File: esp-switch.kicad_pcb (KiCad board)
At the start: 2 copper layers, 51.4 x 51.4 mm, 28 parts, among them J1 Screw_Terminal_01x03, J2 Conn_01x04, J4 Conn_01x04, J5 Screw_Terminal_01x02, U1 ATTINY441-SSU, U2 ESP-01v090, U3 MOC3041M, U4 MOC3041M, U5 HLK-PM05

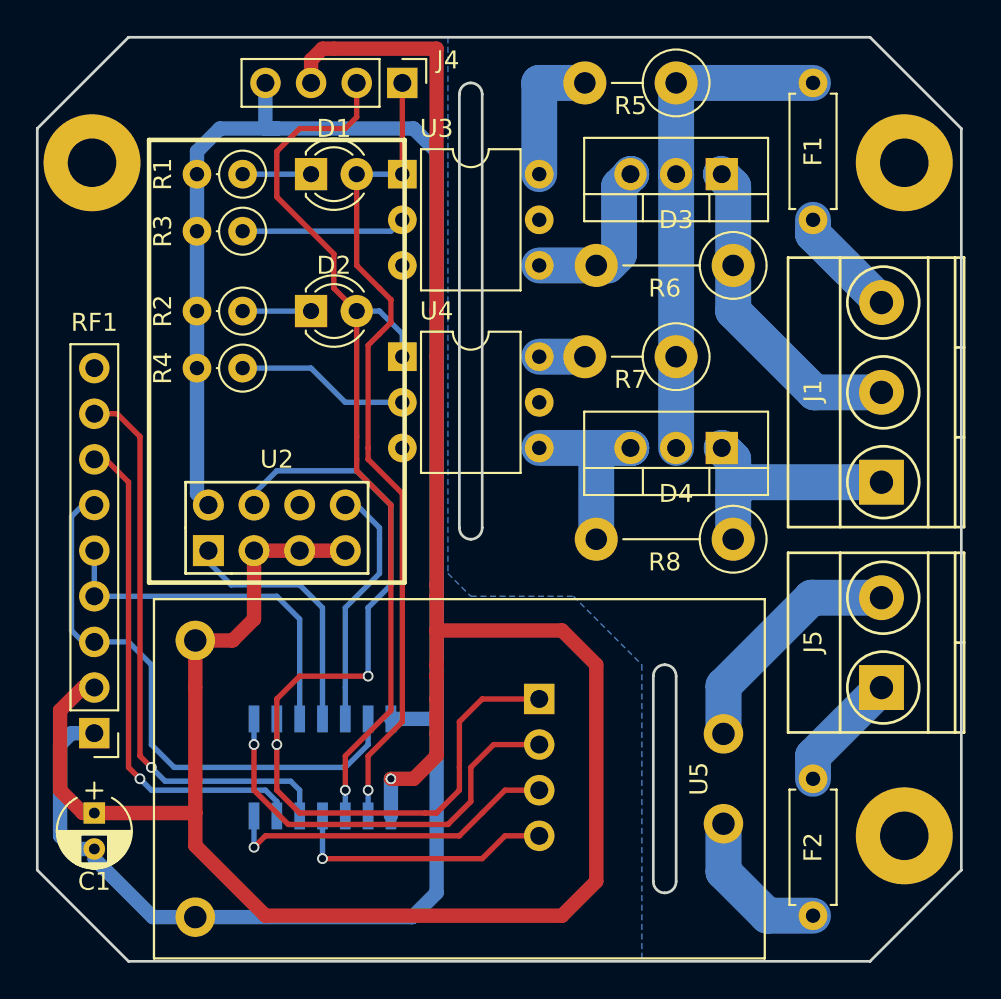
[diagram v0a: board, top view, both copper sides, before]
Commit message: Some changes
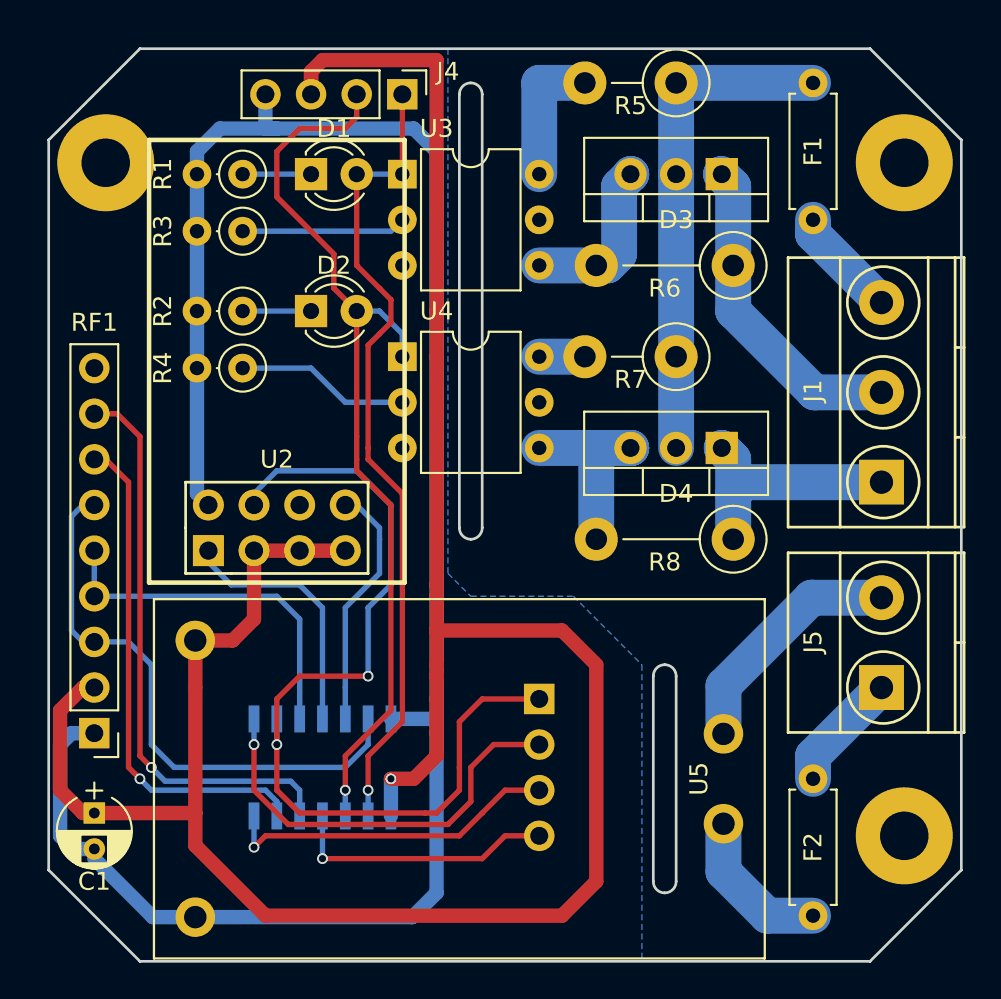
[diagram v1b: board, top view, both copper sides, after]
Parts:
- moved REF** 0.76 mm to (176.5, 99.7)
- moved J4 0.64 mm to (193.0, 95.9)
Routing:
- net Net-(D2-Pad2): track 52.1 -> 51.5 mm
- net Net-(D1-Pad2): track 46.2 -> 45.6 mm
- net GND: track 112.5 -> 111.9 mm
- net +5V: track 139.1 -> 138.5 mm
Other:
- board size 51.4 x 51.4 mm -> 50.8 x 50.8 mm
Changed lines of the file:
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@@
     (area 163.410857 90.20238 240.26 153.195001)
     (thickness 1.6)
-    (drawings 23)
-    (tracks 243)
+    (drawings 21)
+    (tracks 242)
     (zones 0)
     (modules 28)
@@
   )
   (module Mounting_Holes:MountingHole_2.7mm_M2.5_Pad (layer F.Cu)
-    (at 175.768 99.695)
+    (at 176.53 99.695)
     (descr "Mounting Hole 2.7mm, M2.5")
     (tags "mounting hole 2.7mm m2.5")
@@
   )
   (module Pin_Headers:Pin_Header_Straight_1x04_Pitch2.54mm (layer F.Cu)
-    (at 193.04 95.25 270)
+    (at 193.04 95.885 270)
     (descr "Through hole straight pin header, 1x04, 2.54mm pitch, single row")
     (tags "Through hole pin header THT 1x04 2.54mm single row")
@@
   (gr_line (start 196.215 120.015) (end 196.215 95.885) (angle 90) (layer Edge.Cuts) (width 0.15))
   (gr_line (start 197.485 120.015) (end 197.485 95.885) (angle 90) (layer Edge.Cuts) (width 0.15))
-  (gr_line (start 177.8 92.71) (end 219.075 92.71) (angle 90) (layer Edge.Cuts) (width 0.15))
-  (gr_line (start 219.075 144.145) (end 177.8 144.145) (angle 90) (layer Edge.Cuts) (width 0.15))
-  (dimension 51.435 (width 0.3) (layer Dwgs.User)
-    (gr_text "51,435 mm" (at 198.4375 151.845) (layer Dwgs.User)
-      (effects (font (size 1.5 1.5) (thickness 0.3)))
-    )
-    (feature1 (pts (xy 224.155 139.065) (xy 224.155 153.195)))
-    (feature2 (pts (xy 172.72 139.065) (xy 172.72 153.195)))
-    (crossbar (pts (xy 172.72 150.495) (xy 224.155 150.495)))
-    (arrow1a (pts (xy 224.155 150.495) (xy 223.028496 151.081421)))
-    (arrow1b (pts (xy 224.155 150.495) (xy 223.028496 149.908579)))
-    (arrow2a (pts (xy 172.72 150.495) (xy 173.846504 151.081421)))
-    (arrow2b (pts (xy 172.72 150.495) (xy 173.846504 149.908579)))
-  )
-  (gr_line (start 224.155 139.065) (end 224.155 97.79) (angle 90) (layer Edge.Cuts) (width 0.15))
-  (gr_line (start 219.075 92.71) (end 224.155 97.79) (angle 90) (layer Edge.Cuts) (width 0.15))
-  (gr_line (start 172.72 97.79) (end 172.72 139.065) (angle 90) (layer Edge.Cuts) (width 0.15))
-  (gr_line (start 177.8 92.71) (end 172.72 97.79) (angle 90) (layer Edge.Cuts) (width 0.15))
-  (gr_line (start 177.8 144.145) (end 172.72 139.065) (angle 90) (layer Edge.Cuts) (width 0.15))
+  (gr_line (start 178.435 93.345) (end 219.075 93.345) (angle 90) (layer Edge.Cuts) (width 0.15))
+  (gr_line (start 219.075 144.145) (end 178.435 144.145) (angle 90) (layer Edge.Cuts) (width 0.15))
+  (gr_line (start 224.155 139.065) (end 224.155 98.425) (angle 90) (layer Edge.Cuts) (width 0.15))
+  (gr_line (start 219.075 93.345) (end 224.155 98.425) (angle 90) (layer Edge.Cuts) (width 0.15))
+  (gr_line (start 173.355 98.425) (end 173.355 139.065) (angle 90) (layer Edge.Cuts) (width 0.15))
+  (gr_line (start 178.435 93.345) (end 173.355 98.425) (angle 90) (layer Edge.Cuts) (width 0.15))
+  (gr_line (start 178.435 144.145) (end 173.355 139.065) (angle 90) (layer Edge.Cuts) (width 0.15))
   (gr_line (start 224.155 139.065) (end 219.075 144.145) (angle 90) (layer Edge.Cuts) (width 0.15))
-  (dimension 51.435 (width 0.3) (layer Dwgs.User)
-    (gr_text "51.435 mm" (at 233.76 118.4275 90) (layer Dwgs.User)
-      (effects (font (size 1.5 1.5) (thickness 0.3)))
-    )
-    (feature1 (pts (xy 224.155 92.71) (xy 235.11 92.71)))
-    (feature2 (pts (xy 224.155 144.145) (xy 235.11 144.145)))
-    (crossbar (pts (xy 232.41 144.145) (xy 232.41 92.71)))
-    (arrow1a (pts (xy 232.41 92.71) (xy 232.996421 93.836504)))
-    (arrow1b (pts (xy 232.41 92.71) (xy 231.823579 93.836504)))
-    (arrow2a (pts (xy 232.41 144.145) (xy 232.996421 143.018496)))
-    (arrow2b (pts (xy 232.41 144.145) (xy 231.823579 143.018496)))
-  )
   (gr_arc (start 207.645 139.7) (end 207.645 140.335) (angle 90) (layer Edge.Cuts) (width 0.15))
   (gr_arc (start 207.645 139.7) (end 208.28 139.7) (angle 90) (layer Edge.Cuts) (width 0.15))
@@
   (gr_arc (start 196.85 120.015) (end 197.485 120.015) (angle 90) (layer Edge.Cuts) (width 0.15))
   (gr_arc (start 196.85 120.015) (end 196.85 120.65) (angle 90) (layer Edge.Cuts) (width 0.15))
+  (segment (start 194.945 93.98) (end 188.595 93.98) (width 0.8) (layer F.Cu) (net 1))
+  (segment (start 188.595 93.98) (end 187.96 94.615) (width 0.8) (layer F.Cu) (net 1))
+  (segment (start 187.96 94.615) (end 187.96 95.885) (width 0.8) (layer F.Cu) (net 1))
   (segment (start 175.895 135.89) (end 175.26 135.89) (width 0.8) (layer F.Cu) (net 1))
   (segment (start 173.99 130.175) (end 175.26 128.905) (width 0.8) (layer F.Cu) (net 1))
@@
   (segment (start 175.26 128.905) (end 175.895 128.905) (width 0.8) (layer F.Cu) (net 1))
   (segment (start 181.515 135.89) (end 175.895 135.89) (width 0.8) (layer F.Cu) (net 1))
-  (segment (start 187.96 93.98) (end 188.595 93.345) (width 0.8) (layer F.Cu) (net 1))
   (segment (start 187.96 95.25) (end 187.96 94.615) (width 0.8) (layer F.Cu) (net 1))
-  (segment (start 187.96 93.98) (end 187.96 95.25) (width 0.8) (layer F.Cu) (net 1))
-  (segment (start 189.23 93.345) (end 188.595 93.345) (width 0.8) (layer F.Cu) (net 1))
-  (segment (start 194.945 93.345) (end 194.945 125.73) (width 0.8) (layer F.Cu) (net 1))
-  (segment (start 189.23 93.345) (end 194.945 93.345) (width 0.8) (layer F.Cu) (net 1))
+  (segment (start 194.945 93.98) (end 194.945 125.73) (width 0.8) (layer F.Cu) (net 1))
   (segment (start 181.515 126.285) (end 183.595 126.285) (width 0.8) (layer F.Cu) (net 1))
   (segment (start 183.595 126.285) (end 184.785 125.095) (width 0.8) (layer F.Cu) (net 1))
@@
   (via (at 192.405 133.985) (size 0.6) (drill 0.4) (layers F.Cu B.Cu) (net 1))
   (segment (start 181.515 126.285) (end 181.515 126.27) (width 0.8) (layer F.Cu) (net 1))
+  (segment (start 185.42 95.885) (end 185.42 97.79) (width 0.8) (layer B.Cu) (net 2))
   (segment (start 181.61 103.505) (end 181.61 100.33) (width 0.8) (layer B.Cu) (net 2))
   (segment (start 181.61 100.33) (end 181.61 99.06) (width 0.8) (layer B.Cu) (net 2))
@@
   (segment (start 173.99 137.16) (end 173.99 132.08) (width 0.8) (layer B.Cu) (net 2))
   (segment (start 174.72 137.89) (end 173.99 137.16) (width 0.8) (layer B.Cu) (net 2))
-  (segment (start 185.42 95.25) (end 185.42 97.79) (width 0.8) (layer B.Cu) (net 2))
   (segment (start 185.42 97.79) (end 193.675 97.79) (width 0.8) (layer B.Cu) (net 2))
   (segment (start 193.675 97.79) (end 194.945 99.06) (width 0.8) (layer B.Cu) (net 2))
@@
   (segment (start 190.5 118.745) (end 189.865 118.745) (width 0.3) (layer B.Cu) (net 5))
   (segment (start 184.15 100.33) (end 187.96 100.33) (width 0.3) (layer B.Cu) (net 6))
+  (segment (start 193.04 95.885) (end 193.04 100.33) (width 0.3) (layer F.Cu) (net 7))
   (segment (start 191.135 115.57) (end 191.135 116.205) (width 0.3) (layer F.Cu) (net 7))
   (segment (start 191.135 116.205) (end 193.04 118.11) (width 0.3) (layer F.Cu) (net 7))
@@
   (segment (start 191.135 134.62) (end 191.135 132.715) (width 0.3) (layer F.Cu) (net 7))
   (via (at 191.135 134.62) (size 0.6) (drill 0.4) (layers F.Cu B.Cu) (net 7))
-  (segment (start 193.04 95.25) (end 193.04 100.33) (width 0.3) (layer F.Cu) (net 7))
   (segment (start 190.5 100.33) (end 193.04 100.33) (width 0.3) (layer B.Cu) (net 7))
   (segment (start 184.15 107.95) (end 187.96 107.95) (width 0.3) (layer B.Cu) (net 8))
+  (segment (start 190.5 95.885) (end 190.5 97.155) (width 0.3) (layer F.Cu) (net 9))
+  (segment (start 189.23 106.68) (end 189.23 104.775) (width 0.3) (layer F.Cu) (net 9))
+  (segment (start 189.23 106.68) (end 190.5 107.95) (width 0.3) (layer F.Cu) (net 9))
+  (segment (start 189.865 97.79) (end 187.325 97.79) (width 0.3) (layer F.Cu) (net 9))
+  (segment (start 187.325 97.79) (end 186.055 99.06) (width 0.3) (layer F.Cu) (net 9))
+  (segment (start 186.055 99.06) (end 186.055 101.6) (width 0.3) (layer F.Cu) (net 9))
+  (segment (start 186.055 101.6) (end 189.23 104.775) (width 0.3) (layer F.Cu) (net 9))
+  (segment (start 190.5 97.155) (end 189.865 97.79) (width 0.3) (layer F.Cu) (net 9))
   (segment (start 190.5 116.205) (end 190.5 116.84) (width 0.3) (layer F.Cu) (net 9))
   (segment (start 190.5 116.84) (end 192.405 118.745) (width 0.3) (layer F.Cu) (net 9))
@@
   (segment (start 190.5 114.935) (end 190.5 116.205) (width 0.3) (layer F.Cu) (net 9))
   (segment (start 190.5 114.935) (end 190.5 107.95) (width 0.3) (layer F.Cu) (net 9))
-  (segment (start 190.5 95.25) (end 190.5 97.155) (width 0.3) (layer F.Cu) (net 9))
-  (segment (start 190.5 97.155) (end 189.865 97.79) (width 0.3) (layer F.Cu) (net 9))
-  (segment (start 186.055 101.6) (end 189.23 104.775) (width 0.3) (layer F.Cu) (net 9))
-  (segment (start 186.055 99.06) (end 186.055 101.6) (width 0.3) (layer F.Cu) (net 9))
-  (segment (start 187.325 97.79) (end 186.055 99.06) (width 0.3) (layer F.Cu) (net 9))
-  (segment (start 189.865 97.79) (end 187.325 97.79) (width 0.3) (layer F.Cu) (net 9))
   (segment (start 189.865 132.715) (end 189.865 133.35) (width 0.3) (layer F.Cu) (net 9))
   (segment (start 192.405 130.175) (end 189.865 132.715) (width 0.3) (layer F.Cu) (net 9))
-  (segment (start 190.5 107.95) (end 189.23 106.68) (width 0.3) (layer F.Cu) (net 9))
-  (segment (start 189.23 106.68) (end 189.23 104.775) (width 0.3) (layer F.Cu) (net 9))
   (segment (start 189.865 136.05) (end 189.865 134.62) (width 0.3) (layer B.Cu) (net 9))
   (segment (start 189.865 133.35) (end 189.865 134.62) (width 0.3) (layer F.Cu) (net 9))
@@
       (pts
         (xy 195.58 122.555) (xy 196.85 123.825) (xy 202.565 123.825) (xy 206.375 127.635) (xy 206.375 144.145)
-        (xy 177.8 144.145) (xy 172.72 139.065) (xy 172.72 97.79) (xy 177.8 92.71) (xy 195.58 92.71)
+        (xy 178.435 144.145) (xy 173.355 139.065) (xy 173.355 98.425) (xy 178.435 93.345) (xy 195.58 93.345)
       )
     )
